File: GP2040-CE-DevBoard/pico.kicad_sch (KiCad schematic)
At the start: 3 parts, among them U1 Raspbery Pi Pico

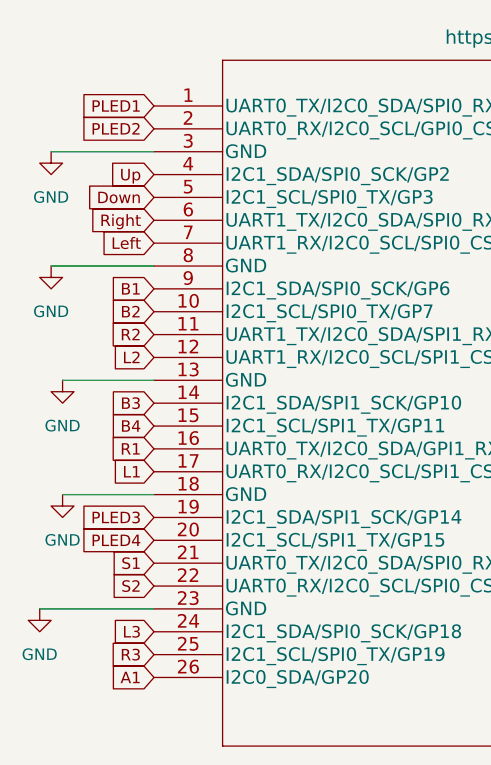
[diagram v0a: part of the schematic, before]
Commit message: Progress
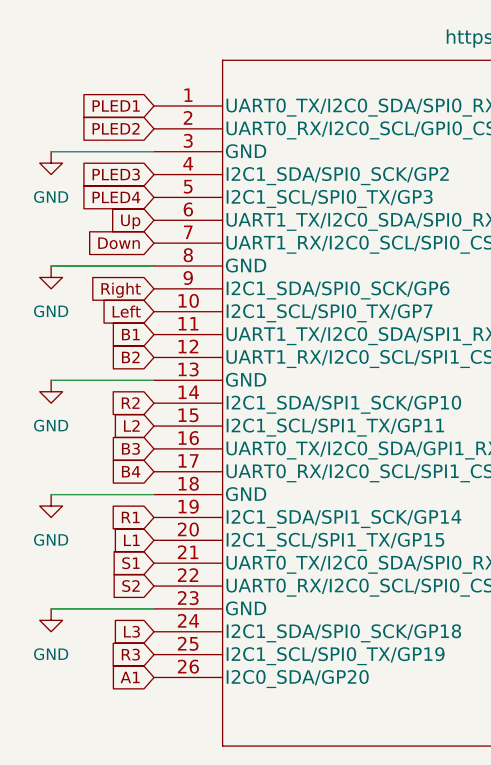
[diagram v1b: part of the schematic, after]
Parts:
- U1: footprint ul_SC0915:SC0915 -> OpenStick:Raspberry Pi Pico - pogo pin and screw mount
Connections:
- net B1: now also U1.11 (UART1_TX/I2C0_SDA/SPI1_RX/GP8); no longer U1.9 (I2C1_SDA/SPI0_SCK/GP6)
- net B2: now also U1.12 (UART1_RX/I2C0_SCL/SPI1_CSn/GP9); no longer U1.10 (I2C1_SCL/SPI0_TX/GP7)
- net B3: now also U1.16 (UART0_TX/I2C0_SDA/GPI1_RX/GP12); no longer U1.14 (I2C1_SDA/SPI1_SCK/GP10)
- net B4: now also U1.17 (UART0_RX/I2C0_SCL/SPI1_CSn/GP13); no longer U1.15 (I2C1_SCL/SPI1_TX/GP11)
- net Down: now also U1.7 (UART1_RX/I2C0_SCL/SPI0_CSn/GP5); no longer U1.5 (I2C1_SCL/SPI0_TX/GP3)
- net L1: now also U1.20 (I2C1_SCL/SPI1_TX/GP15); no longer U1.17 (UART0_RX/I2C0_SCL/SPI1_CSn/GP13)
- net L2: now also U1.15 (I2C1_SCL/SPI1_TX/GP11); no longer U1.12 (UART1_RX/I2C0_SCL/SPI1_CSn/GP9)
- net Left: now also U1.10 (I2C1_SCL/SPI0_TX/GP7); no longer U1.7 (UART1_RX/I2C0_SCL/SPI0_CSn/GP5)
- net PLED3: now also U1.4 (I2C1_SDA/SPI0_SCK/GP2); no longer U1.19 (I2C1_SDA/SPI1_SCK/GP14)
- net PLED4: now also U1.5 (I2C1_SCL/SPI0_TX/GP3); no longer U1.20 (I2C1_SCL/SPI1_TX/GP15)
- net R1: now also U1.19 (I2C1_SDA/SPI1_SCK/GP14); no longer U1.16 (UART0_TX/I2C0_SDA/GPI1_RX/GP12)
- net R2: now also U1.14 (I2C1_SDA/SPI1_SCK/GP10); no longer U1.11 (UART1_TX/I2C0_SDA/SPI1_RX/GP8)
- net Right: now also U1.9 (I2C1_SDA/SPI0_SCK/GP6); no longer U1.6 (UART1_TX/I2C0_SDA/SPI0_RX/GP4)
- net Up: now also U1.6 (UART1_TX/I2C0_SDA/SPI0_RX/GP4); no longer U1.4 (I2C1_SDA/SPI0_SCK/GP2)

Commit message: a lot of Silkscreen work
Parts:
- R3, R4: footprint Capacitor_SMD:C_0805_2012Metric_Pad1.18x1.45mm_HandSolder -> OpenStick:C_0805_2012Metric_Pad1.18x1.45mm_HandSolder
- U1: footprint OpenStick:Raspberry Pi Pico - pogo pin and screw mount -> ul_SC0915:Pico
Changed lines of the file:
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@@
       (effects (font (size 1.524 1.524)))
     )
-    (property "Footprint" "OpenStick:Raspberry Pi Pico - pogo pin and screw mount" (id 2) (at 149.86 40.894 0)
+    (property "Footprint" "ul_SC0915:Pico" (id 2) (at 149.86 40.894 0)
       (effects (font (size 1.524 1.524)) hide)
     )
@@
       (effects (font (size 1.27 1.27)) (justify left))
     )
-    (property "Footprint" "Capacitor_SMD:C_0805_2012Metric_Pad1.18x1.45mm_HandSolder" (id 2) (at 234.442 106.68 90)
+    (property "Footprint" "OpenStick:C_0805_2012Metric_Pad1.18x1.45mm_HandSolder" (id 2) (at 234.442 106.68 90)
       (effects (font (size 1.27 1.27)) hide)
     )
@@
   (symbol (lib_id "power:GND") (at 74.93 102.87 0) (unit 1)
     (in_bom yes) (on_board yes) (fields_autoplaced)
-    (property "Reference" "#PWR07" (id 0) (at 74.93 109.22 0)
+    (property "Reference" "#PWR011" (id 0) (at 74.93 109.22 0)
       (effects (font (size 1.27 1.27)) hide)
     )
@@
   (symbol (lib_id "power:GND") (at 74.93 77.47 0) (unit 1)
     (in_bom yes) (on_board yes) (fields_autoplaced)
-    (property "Reference" "#PWR010" (id 0) (at 74.93 83.82 0)
+    (property "Reference" "#PWR09" (id 0) (at 74.93 83.82 0)
       (effects (font (size 1.27 1.27)) hide)
     )
@@
       (effects (font (size 1.27 1.27)) (justify left))
     )
-    (property "Footprint" "Capacitor_SMD:C_0805_2012Metric_Pad1.18x1.45mm_HandSolder" (id 2) (at 225.552 109.22 90)
+    (property "Footprint" "OpenStick:C_0805_2012Metric_Pad1.18x1.45mm_HandSolder" (id 2) (at 225.552 109.22 90)
       (effects (font (size 1.27 1.27)) hide)
     )
@@
   (symbol (lib_id "power:GND") (at 74.93 52.07 0) (unit 1)
     (in_bom yes) (on_board yes) (fields_autoplaced)
-    (property "Reference" "#PWR08" (id 0) (at 74.93 58.42 0)
+    (property "Reference" "#PWR07" (id 0) (at 74.93 58.42 0)
       (effects (font (size 1.27 1.27)) hide)
     )
@@
   (symbol (lib_id "power:GND") (at 74.93 90.17 0) (unit 1)
     (in_bom yes) (on_board yes) (fields_autoplaced)
-    (property "Reference" "#PWR011" (id 0) (at 74.93 96.52 0)
+    (property "Reference" "#PWR010" (id 0) (at 74.93 96.52 0)
       (effects (font (size 1.27 1.27)) hide)
     )
@@
   (symbol (lib_id "power:GND") (at 74.93 64.77 0) (unit 1)
     (in_bom yes) (on_board yes) (fields_autoplaced)
-    (property "Reference" "#PWR09" (id 0) (at 74.93 71.12 0)
-      (effects (font (size 1.27 1.27)) hide)
-    )
+    (property "Reference" "#PWR08" (id 0) (at 74.93 71.12 0)
+      (effects (font (size 1.27 1.27)) hide)
+    )
